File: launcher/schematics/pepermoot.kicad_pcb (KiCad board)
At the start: 2 copper layers, 83 x 119 mm, 20 parts, among them J3 Power, J4 Dispenser motor, J7 Extra, J8 Pul motor, J9 End switch (1,2) , Servo (3,4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, U2 ESP32-DevKitC

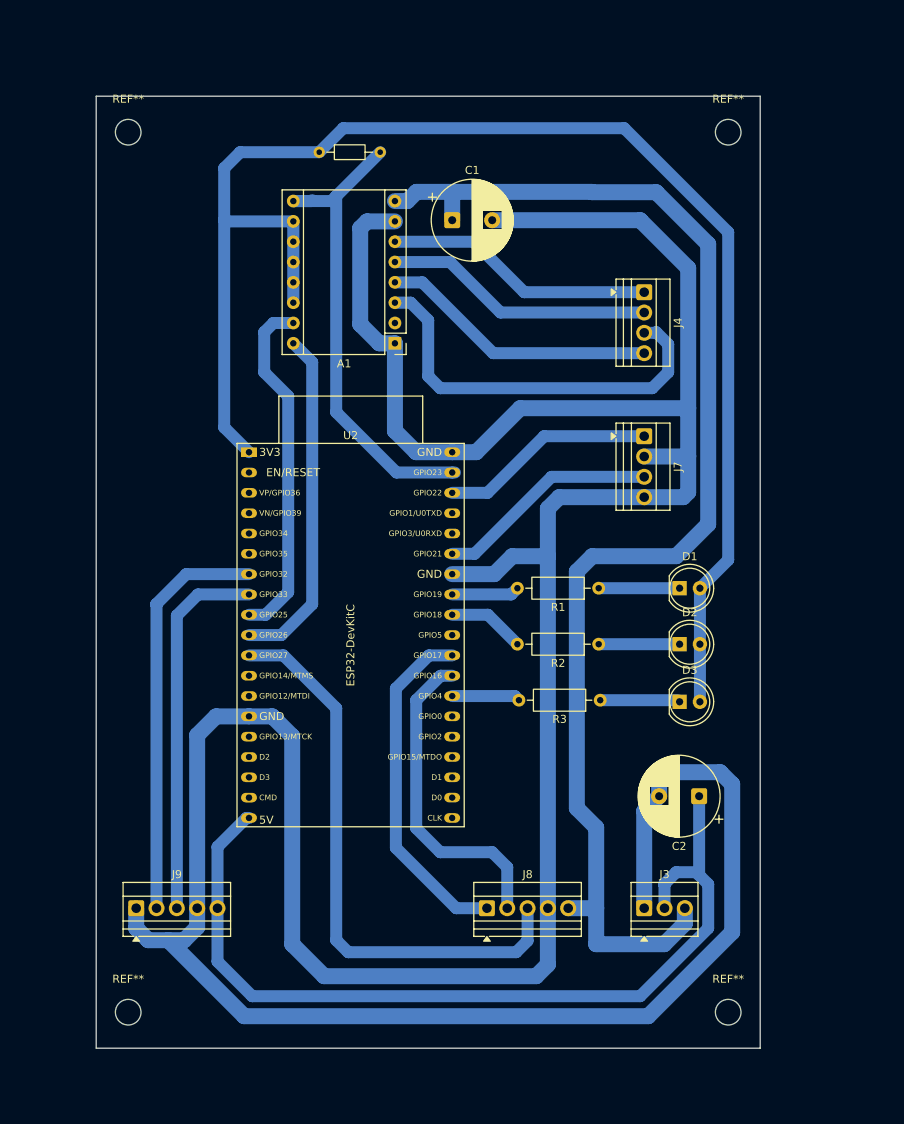
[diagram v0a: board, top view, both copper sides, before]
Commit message: pcb update
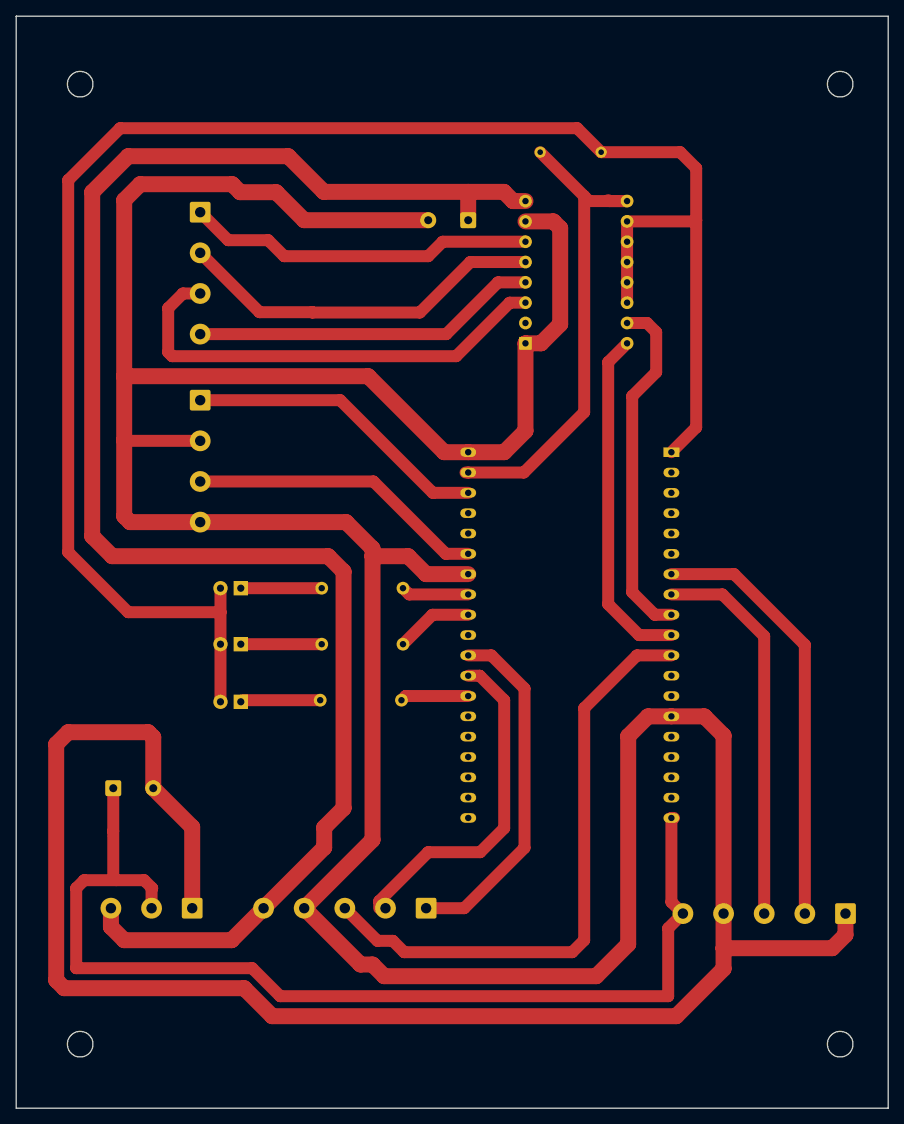
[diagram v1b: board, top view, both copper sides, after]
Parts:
- A1, C1, C2, D1, D2, D3, R1, R2, R3, R4, REF** (x4), U2: moved to B.Cu
- J3: footprint TerminalBlock:TerminalBlock_Xinya_XY308-2.54-3P_1x03_P2.54mm_Horizontal -> TerminalBlock_Phoenix:TerminalBlock_Phoenix_MKDS-1,5-3-5.08_1x03_P5.08mm_Horizontal; moved to B.Cu
- J4, J7: footprint TerminalBlock:TerminalBlock_Xinya_XY308-2.54-4P_1x04_P2.54mm_Horizontal -> TerminalBlock_Phoenix:TerminalBlock_Phoenix_MKDS-1,5-4-5.08_1x04_P5.08mm_Horizontal; moved to B.Cu
- J8, J9: footprint TerminalBlock:TerminalBlock_Xinya_XY308-2.54-5P_1x05_P2.54mm_Horizontal -> TerminalBlock_Phoenix:TerminalBlock_Phoenix_MKDS-1,5-5-5.08_1x05_P5.08mm_Horizontal; moved to B.Cu
- moved REF** 89.2 mm to (145.0, 30.0), turned to 180 degrees
- moved REF** 89.1 mm to (145.0, 150.0), turned to 180 degrees
- moved J9 88.7 mm to (145.7, 133.7), turned to 180 degrees
- moved REF** 81.2 mm to (50.0, 30.0), turned to 180 degrees
- moved REF** 81.1 mm to (50.0, 150.0), turned to 180 degrees
- moved C2 73.2 mm to (54.1, 118.0), turned to 0 degrees
- moved J3 56.5 mm to (64.0, 133.0), turned to 180 degrees
- moved J4 56.4 mm to (65.0, 46.0)
- moved J7 55.7 mm to (65.0, 69.5)
- moved D1 54.8 mm to (70.1, 93.0), turned to 180 degrees
- moved D2 54.8 mm to (70.1, 100.0), turned to 180 degrees
- moved D3 54.8 mm to (70.1, 107.2), turned to 180 degrees
- moved U2 52.8 mm to (123.9, 76.0), turned to 180 degrees
- moved R4 35.2 mm to (115.1, 38.5), turned to 180 degrees
- moved R3 35.0 mm to (80.0, 107.0), turned to 0 degrees
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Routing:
- net GND: track 455.7 -> 559.0 mm
- net +24V: track 164.9 -> 208.1 mm
- net Net-(A1-M0): track 186.3 -> 221.8 mm
- net +5V: track 111.5 -> 134.8 mm
- net Net-(A1-B1): track 33.8 -> 46.4 mm
- net Net-(J7-Pin_1): track 26.9 -> 38.3 mm
- net Net-(A1-B2): track 33.8 -> 43.7 mm
- net Net-(J7-Pin_3): track 28.0 -> 37.2 mm
- net Net-(A1-A1): track 34.8 -> 43.3 mm
- net Net-(A1-A2): track 50.7 -> 57.9 mm
- net Net-(J8-Pin_3): track 71.8 -> 75.5 mm
- net Net-(J9-Pin_2): track 51.2 -> 53.9 mm
- net Net-(J8-Pin_2): track 40.3 -> 42.0 mm
- net Net-(J9-Pin_3): track 46.7 -> 48.4 mm
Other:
- board size 83 x 119 mm -> 109 x 136.5 mm
